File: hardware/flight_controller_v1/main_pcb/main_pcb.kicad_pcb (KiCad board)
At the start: 2 copper layers, 50.8 x 50.8 mm, 20 parts, among them M1 Conn_01x03, M2 Conn_01x03, M3 Conn_01x03, M4 Conn_01x03, U1 CH340E, U2 ICM-20948, U3 TLV70018_SOT23-5, U5 L78L33_SOT89, U7 NEO-M8N, U8 ESP32-WROOM-32U

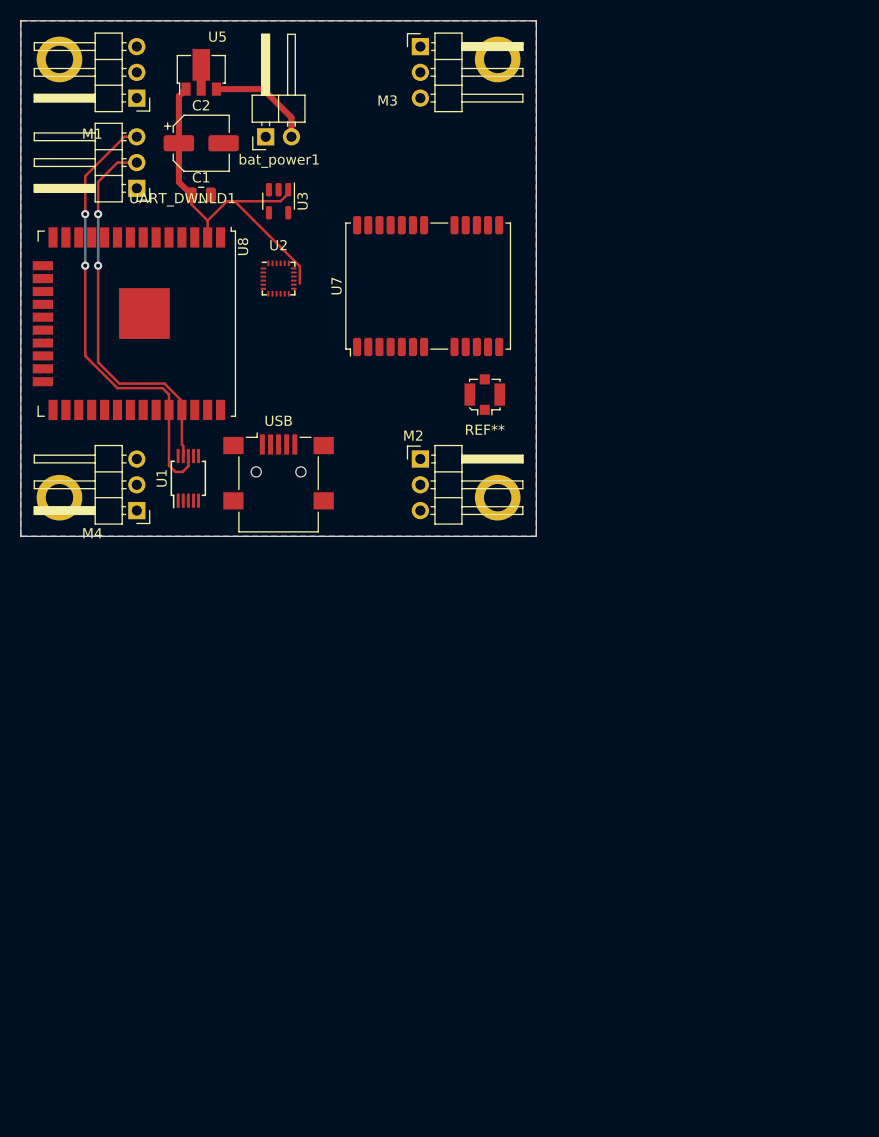
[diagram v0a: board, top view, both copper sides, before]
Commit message: New PCB iteration
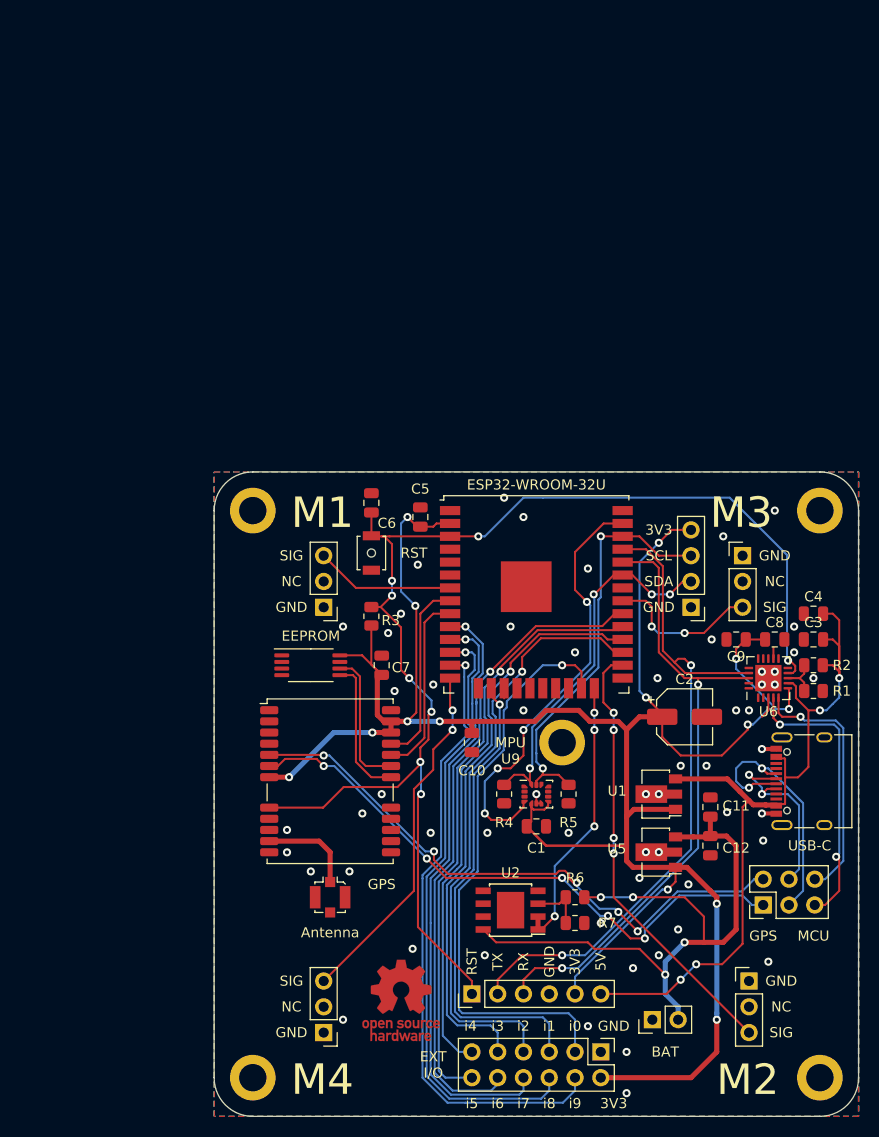
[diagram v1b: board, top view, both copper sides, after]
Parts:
- removed U3: TLV70018_SOT23-5, Package_TO_SOT_SMD:SOT-23-5
- removed UART_DWNLD1: Conn_01x03, Connector_PinHeader_2.54mm:PinHeader_1x03_P2.54mm_Horizontal
- removed USB: USB, Connector_USB:USB_Mini-B_Lumberg_2486_01_Horizontal
- added ?: , , F.Cu at (154.9, 96.5)
- added C10: 0.1uF, Capacitor_SMD:C_0805_2012Metric, F.Cu at (146.1, 96.5)
- added C11: 10uF, Capacitor_SMD:C_0805_2012Metric, F.Cu at (169.5, 102.9)
- added C12: 0.1uF, Capacitor_SMD:C_0805_2012Metric, F.Cu at (169.5, 106.7)
- added C3: 4.7uF, Capacitor_SMD:C_0805_2012Metric, F.Cu at (179.7, 86.4)
- added C4: 0.1uF, Capacitor_SMD:C_0805_2012Metric, F.Cu at (179.7, 83.8)
- added C5: 0.1uF, Capacitor_SMD:C_0805_2012Metric, F.Cu at (141.0, 74.3)
- added C6: 1uF, Capacitor_SMD:C_0805_2012Metric, F.Cu at (136.1, 72.9)
- added C7: 0.1uF, Capacitor_SMD:C_0805_2012Metric, F.Cu at (137.2, 88.9)
- added C8: 4.7uF, Capacitor_SMD:C_0805_2012Metric, F.Cu at (175.9, 86.4)
- added C9: 0.1uF, Capacitor_SMD:C_0805_2012Metric, F.Cu at (172.1, 86.4)
- added EEPROM1: 24LC32, Package_SO:TSSOP-8_4.4x3mm_P0.65mm, F.Cu at (130.2, 88.9)
- added J1: Conn_01x06, Connector_PinHeader_2.54mm:PinHeader_1x06_P2.54mm_Vertical, F.Cu at (146.1, 121.3)
- added J2: Conn_01x04_Female, Connector_PinHeader_2.54mm:PinHeader_1x04_P2.54mm_Vertical, F.Cu at (167.6, 83.2)
- added J3: Conn_02x06_Counter_Clockwise, Connector_PinHeader_2.54mm:PinHeader_2x06_P2.54mm_Vertical, F.Cu at (158.8, 127.0)
- added J4: Conn_02x03_Odd_Even, Connector_PinHeader_2.54mm:PinHeader_2x03_P2.54mm_Vertical, F.Cu at (174.8, 112.5)
- added R1: 22.1k, Resistor_SMD:R_0805_2012Metric, F.Cu at (179.7, 88.9)
- added R2: 47.5k, Resistor_SMD:R_0805_2012Metric, F.Cu at (179.7, 91.4)
- added R3: 10k, Resistor_SMD:R_0805_2012Metric, F.Cu at (136.1, 84.1)
- added R4: 10k, Resistor_SMD:R_0805_2012Metric, F.Cu at (149.2, 101.6)
- added R5: 10k, Resistor_SMD:R_0805_2012Metric, F.Cu at (155.6, 101.6)
- added R6: 3M, Resistor_SMD:R_0805_2012Metric, F.Cu at (156.2, 111.8)
- added R7: 1M, Resistor_SMD:R_0805_2012Metric, F.Cu at (156.2, 114.3)
- added REF**: OSHW-Logo_7.5x8mm_Copper, Symbol:OSHW-Logo_7.5x8mm_Copper, F.Cu at (139.1, 121.9)
- added SW1: SW_Push, Button_Switch_SMD:SW_SPST_B3U-1000P-B, F.Cu at (136.1, 77.8)
- added U6: CP2102N-Axx-xQFN20, Package_DFN_QFN:MLF-20-1EP_4x4mm_P0.5mm_EP2.6x2.6mm, F.Cu at (175.3, 90.2)
- added U9: LSM6DS3, Package_LGA:LGA-14_3x2.5mm_P0.5mm_LayoutBorder3x4y, F.Cu at (152.4, 101.6)
- added USB-C: USB_C_Receptacle_XKB_U262-16XN-4BVC11, Connector_USB:USB_C_Receptacle_XKB_U262-16XN-4BVC11, F.Cu at (179.7, 100.3)
- BAT1: renamed from bat_power1; footprint Connector_PinHeader_2.54mm:PinHeader_1x02_P2.54mm_Horizontal -> Connector_PinHeader_2.54mm:PinHeader_1x02_P2.54mm_Vertical
- C2: footprint Capacitor_SMD:CP_Elec_5x3 -> Capacitor_SMD:CP_Elec_5x4.5
- M1, M2, M3, M4: footprint Connector_PinHeader_2.54mm:PinHeader_1x03_P2.54mm_Horizontal -> Connector_PinHeader_2.54mm:PinHeader_1x03_P2.54mm_Vertical
- U1: value CH340E -> L78L33_SOT89; footprint Package_SO:MSOP-10_3x3mm_P0.5mm -> Package_TO_SOT_SMD:SOT-89-3
- U2: value ICM-20948 -> LM2904; footprint Sensor_Motion:InvenSense_QFN-24_3x3mm_P0.4mm -> Package_SO:Diodes_PSOP-8
- moved BAT1 95.0 mm to (163.8, 123.8)
- moved U5 89.1 mm to (164.5, 107.3), turned to 180 degrees
- moved C2 73.9 mm to (167.0, 94.0)
- moved C1 70.4 mm to (152.4, 104.8)
- moved U2 66.3 mm to (149.9, 113.0), turned to 180 degrees
- moved ? 65.4 mm to (180.3, 129.5)
- moved M2 60.8 mm to (173.4, 120.0)
- moved ? 60.2 mm to (124.5, 129.5)
- moved M3 59.4 mm to (172.7, 78.1)
- moved U1 55.8 mm to (164.5, 101.6), turned to 180 degrees
- moved M4 54.6 mm to (131.4, 125.1)
- moved ? 54.6 mm to (180.3, 73.7)
- moved M1 53.4 mm to (131.4, 83.2)
- moved Antenna 51.8 mm to (132.1, 111.8), turned to 180 degrees
- moved GPS1 49.7 mm to (132.1, 100.3), turned to 0 degrees
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- renumbered REF** to Antenna, U8 to ESP32-WROOM-32U1, U7 to GPS1
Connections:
- Antenna pad 1: (no net) -> /gps_antenna
- ESP32-WROOM-32U1 pad 10: unconnected-(U8-Pad10) -> xIO3
- ESP32-WROOM-32U1 pad 11: unconnected-(U8-Pad11) -> xIO2
- ESP32-WROOM-32U1 pad 12: unconnected-(U8-Pad12) -> xIO1
- ESP32-WROOM-32U1 pad 13: unconnected-(U8-Pad13) -> xIO6
- ESP32-WROOM-32U1 pad 14: unconnected-(U8-Pad14) -> M4
- ESP32-WROOM-32U1 pad 16: unconnected-(U8-Pad16) -> xIO4
- ESP32-WROOM-32U1 pad 23: unconnected-(U8-Pad23) -> xIO5
- ESP32-WROOM-32U1 pad 24: unconnected-(U8-Pad24) -> VBAT_LL
- ESP32-WROOM-32U1 pad 26: unconnected-(U8-Pad26) -> M2
- ESP32-WROOM-32U1 pad 27: unconnected-(U8-Pad27) -> xIO7
- ESP32-WROOM-32U1 pad 28: unconnected-(U8-Pad28) -> xIO8
- ESP32-WROOM-32U1 pad 29: unconnected-(U8-Pad29) -> xIO10
- ESP32-WROOM-32U1 pad 3: unconnected-(U8-Pad3) -> RESET
- ESP32-WROOM-32U1 pad 30: unconnected-(U8-Pad30) -> xIO9
- ESP32-WROOM-32U1 pad 31: unconnected-(U8-Pad31) -> M3
- ESP32-WROOM-32U1 pad 33: unconnected-(U8-Pad33) -> SDA
- ESP32-WROOM-32U1 pad 36: unconnected-(U8-Pad36) -> SCL
- ESP32-WROOM-32U1 pad 37: unconnected-(U8-Pad37) -> MPU_INT_1
- ESP32-WROOM-32U1 pad 6: unconnected-(U8-Pad6) -> xIO6
- ESP32-WROOM-32U1 pad 7: unconnected-(U8-Pad7) -> M1
- ESP32-WROOM-32U1 pad 8: unconnected-(U8-Pad8) -> GPS_RX
- ESP32-WROOM-32U1 pad 9: unconnected-(U8-Pad9) -> GPS_TX
- GPS1 pad 10: Net-(U7-Pad10) -> GND
- GPS1 pad 11: unconnected-(U7-Pad11) -> /gps_antenna
- GPS1 pad 12: Net-(U7-Pad10) -> GND
- GPS1 pad 13: Net-(U7-Pad10) -> GND
- GPS1 pad 18: unconnected-(U7-Pad18) -> SDA_eeprom
- GPS1 pad 19: unconnected-(U7-Pad19) -> SCL_eeprom
- GPS1 pad 20: unconnected-(U7-Pad20) -> GPS_TX
- GPS1 pad 21: unconnected-(U7-Pad21) -> GPS_RX
- GPS1 pad 22: unconnected-(U7-Pad22) -> +3V3
- GPS1 pad 23: unconnected-(U7-Pad23) -> +3V3
- GPS1 pad 24: Net-(U7-Pad10) -> GND
- GPS1 pad 5: unconnected-(U7-Pad5) -> USB-gps
- GPS1 pad 6: unconnected-(U7-Pad6) -> USB+gps
- GPS1 pad 8: unconnected-(U7-Pad8) -> RESET
- U1 pad 1: USB+ -> +3V3
- U1 pad 2: USB- -> GND
- U1 pad 3: GND -> USB5V
- U2 pad 1: unconnected-(U2-Pad1) -> VBAT_LL
- U2 pad 2: unconnected-(U2-Pad2) -> VBAT_LL
- U2 pad 3: unconnected-(U2-Pad3) -> Net-(R6-Pad2)
- U2 pad 4: unconnected-(U2-Pad4) -> GND
- U2 pad 8: +1V8 -> v_bat
- U2 pad 9: unconnected-(U2-Pad9) -> (no net)
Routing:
- net +3V3: track 37.0 -> 229.6 mm, vias 0 -> 14
- net RESET: track 0.00 -> 128.6 mm, vias 0 -> 8
- net USB5V: track 0.00 -> 80.7 mm, vias 0 -> 4
- net xIO6: track 0.00 -> 62.0 mm, vias 0 -> 1
- net xIO1: track 0.00 -> 60.8 mm, vias 0 -> 1
- net xIO9: track 0.00 -> 60.6 mm, vias 0 -> 1
- net xIO7: track 0.00 -> 59.7 mm, vias 0 -> 1
- net USB-gps: track 0.00 -> 59.2 mm, vias 0 -> 5
- net xIO2: track 0.00 -> 58.9 mm, vias 0 -> 1
- net USB+gps: track 0.00 -> 58.9 mm, vias 0 -> 5
- net xIO5: track 0.00 -> 58.1 mm, vias 0 -> 1
- net xIO8: track 0.00 -> 57.6 mm, vias 0 -> 1
- net xIO3: track 0.00 -> 56.4 mm, vias 0 -> 1
- net xIO10: track 0.00 -> 56.1 mm, vias 0 -> 1
- net v_bat: track 10.5 -> 66.0 mm, vias 0 -> 4
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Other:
- board size 50.8 x 50.8 mm -> 63.5 x 63.5 mm
- board text added: "3V3"
- board text added: "5V"
- board text added: "BAT"
- board text added: "EEPROM"
- board text added: "ESP32-WROOM-32U"
- board text added: "EXT I/O"
- board text added: "GND"
- board text added: "GPS"
- board text added: "MCU"
- board text added: "MPU"
- board text added: "NC"
- board text added: "Project :"
- board text added: "RST"
- board text added: "RX"
- board text added: "SCL"
- board text added: "SDA"
- board text added: "SIG"
- board text added: "TX"
- board text added: "by Peter Krull"
- board text added: "i0"
- board text added: "i1"
- board text added: "i2"
- board text added: "i3"
- board text added: "i4"
- board text added: "i5"
- board text added: "i6"
- board text added: "i7"
- board text added: "i8"
- board text added: "i9"
- board text added: "quad v0.1"
